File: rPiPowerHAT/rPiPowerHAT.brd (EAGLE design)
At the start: 80 x 100 mm, 3 parts, among them X1 MKDSN1,5/2-5,08, X2 MKDSN1,5/2-5,08

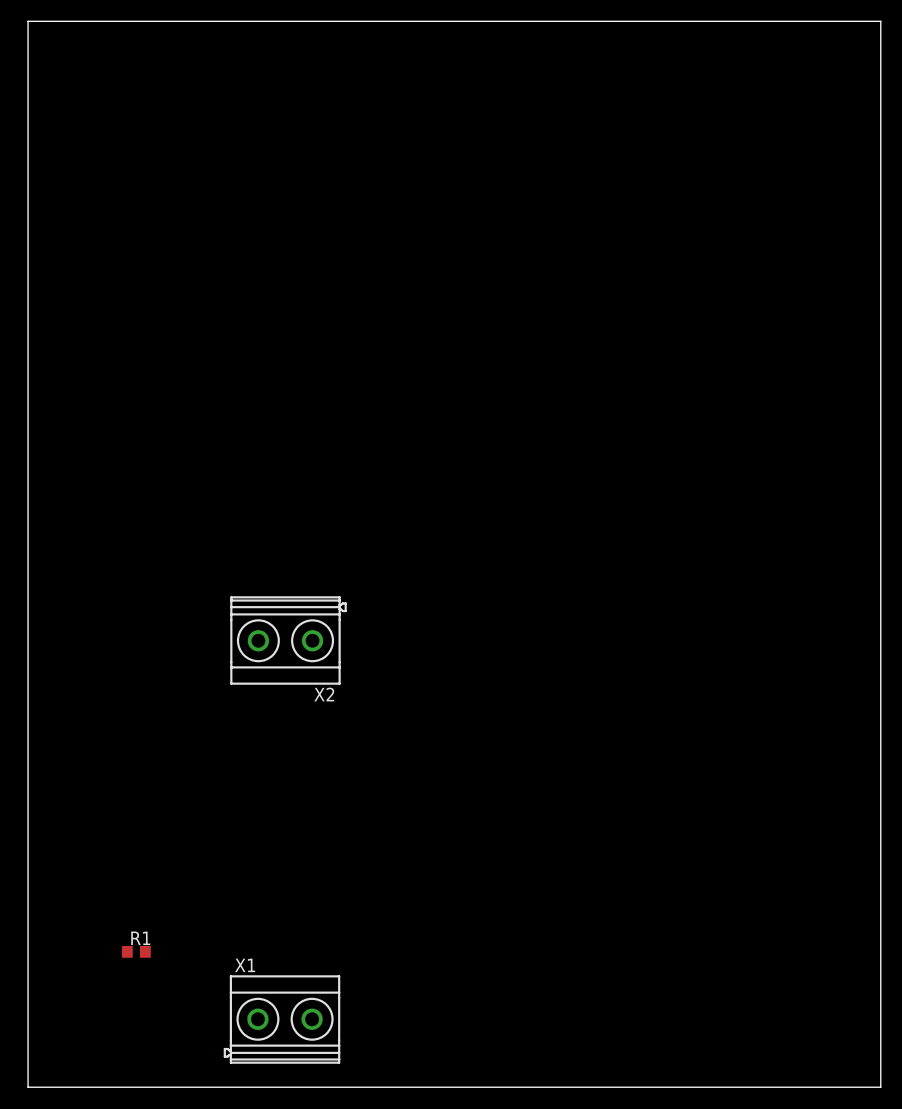
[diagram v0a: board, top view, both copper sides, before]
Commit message: .
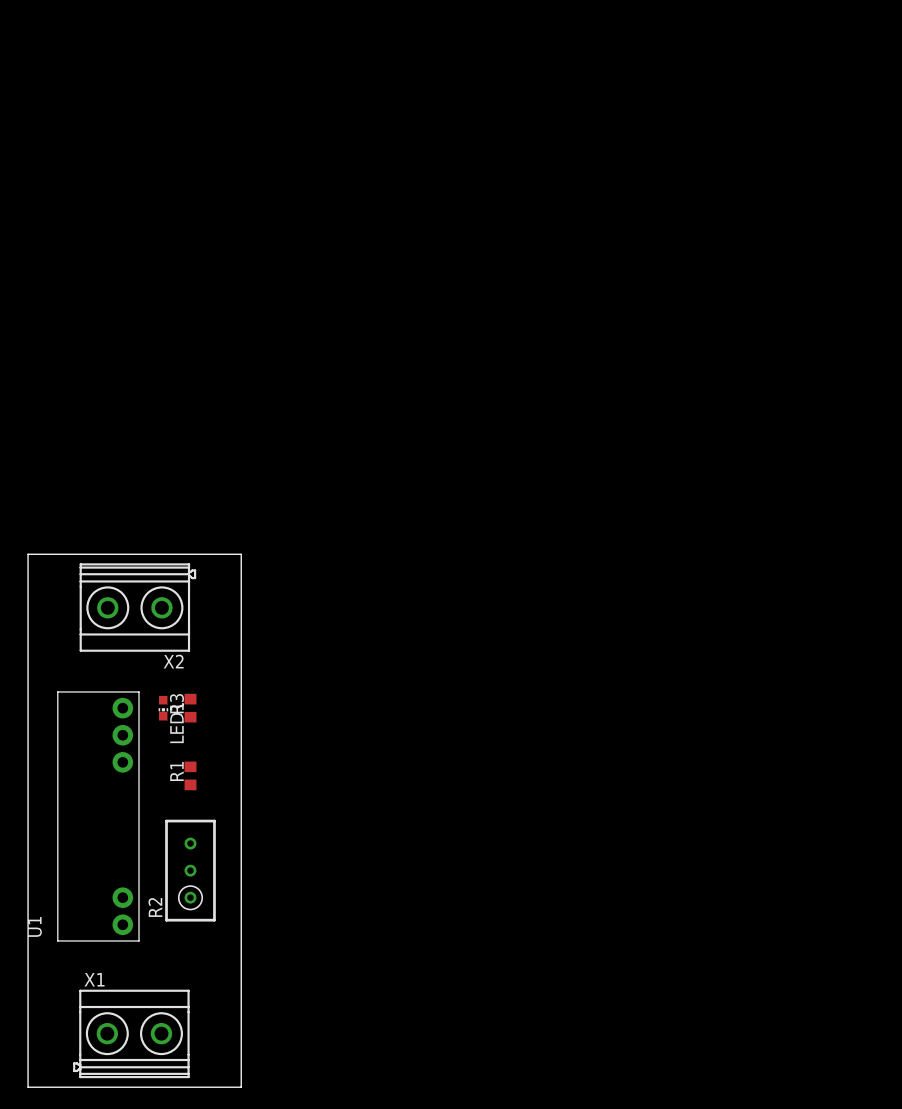
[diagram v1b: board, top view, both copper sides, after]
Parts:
- added LED1: (no value), adafruit:CHIP-LED0603
- added R2: 1k, hojunsong:RTRIM3296W
- added R3: 1k, rcl:R0603
- added U1: OKX-T/3-D12, hojunsong:OKX-T/3-D12
- moved R1 17.3 mm to (15.2, 29.2), turned to 90 degrees
- moved X2 14.5 mm to (10.0, 45.0)
- moved X1 14.2 mm to (10.0, 5.00)
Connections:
- new net N$1: R1.2, U1.2
- new net N$2: R1.1, R2.3
- new net N$3: LED1.C, R3.2
- net +12V: now also U1.4
- net +5V: now also LED1.A, U1.1
- net GND: now also R2.2, R3.1, U1.3
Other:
- board size 80 x 100 mm -> 20 x 50 mm
